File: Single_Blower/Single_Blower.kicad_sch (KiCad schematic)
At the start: 15 parts, among them J1 BLOWER, J3 LED, J4 Sensor Connection, J5 LIMIT Switch, J6 DE9_Pins_MountingHoles, U2 5V

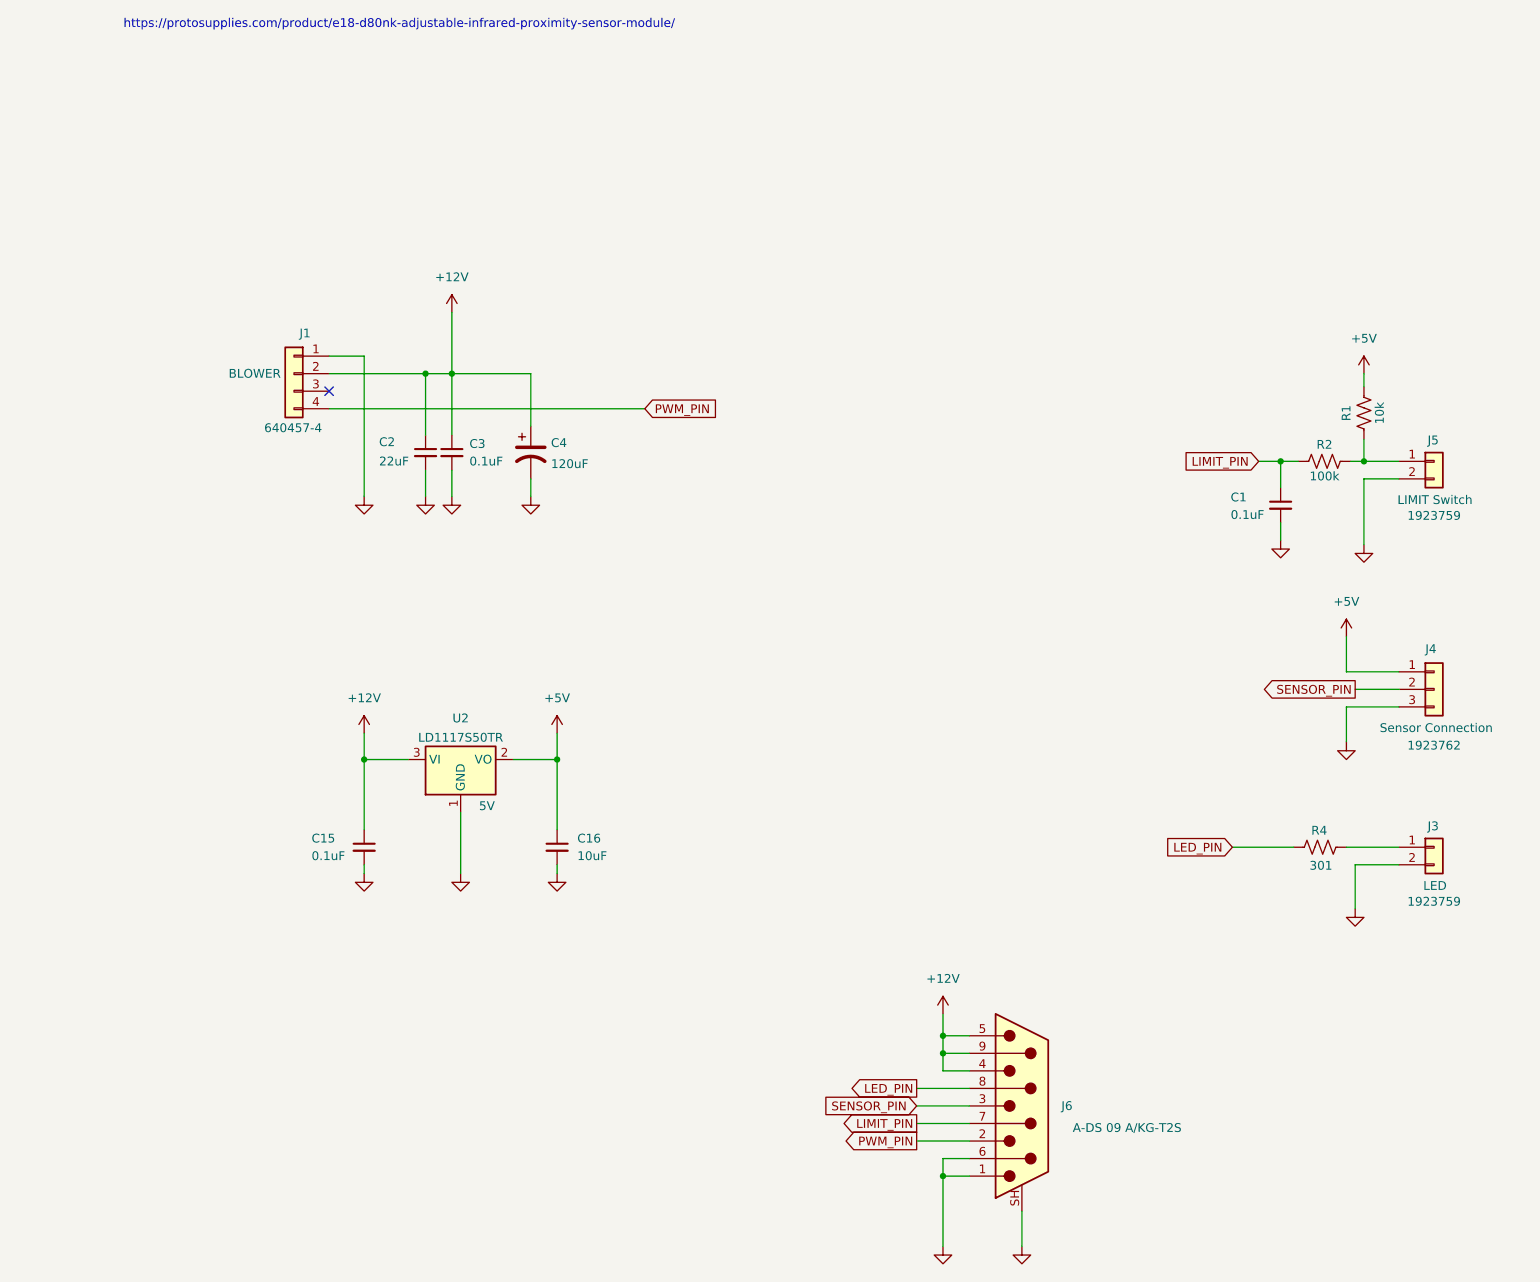
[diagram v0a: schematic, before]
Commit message: board layout
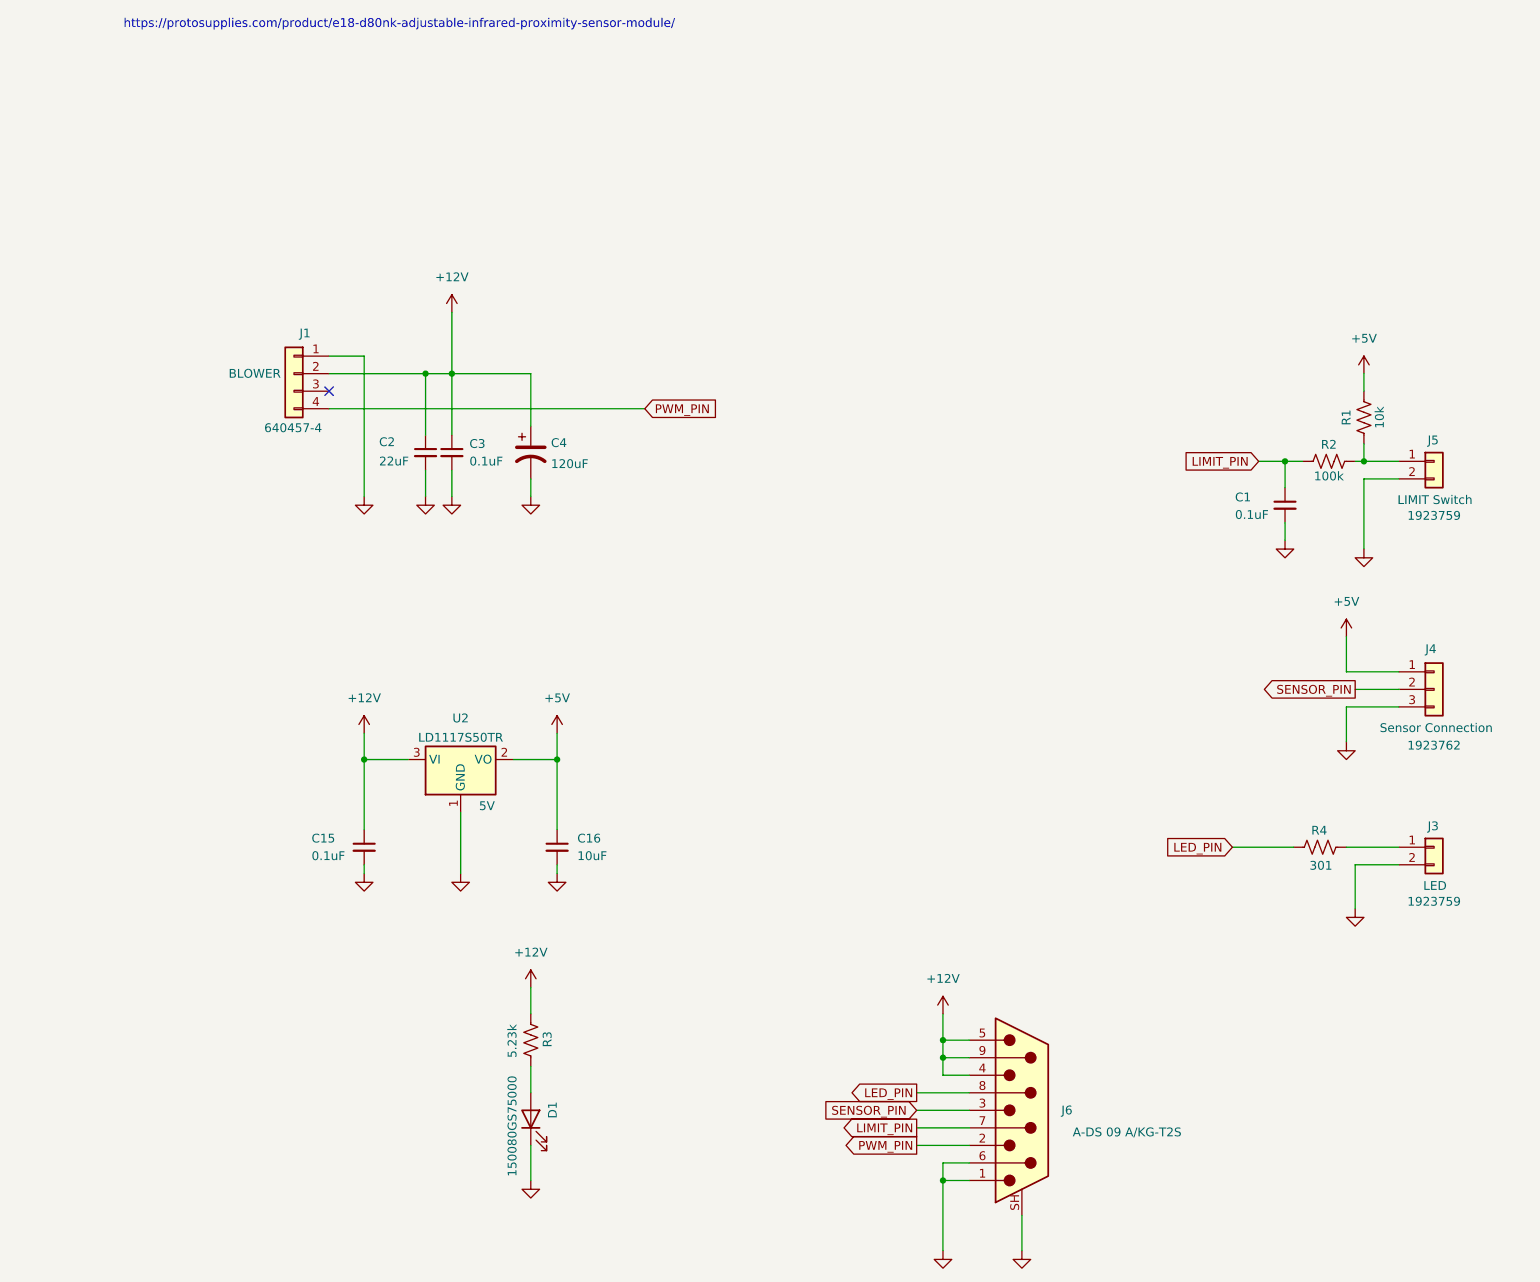
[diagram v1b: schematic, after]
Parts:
- added D1: PWR, LED_SMD:LED_0805_2012Metric, symbol Device:LED
- added R3: 5.23k, Resistor_SMD:R_0805_2012Metric, symbol Device:R_US
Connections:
- net +12V: now also R3.1
- net GND: now also D1.1 (K)
- new net: D1.2 (A), R3.2
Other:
- moved on the sheet: C1, J6, R1, R2
